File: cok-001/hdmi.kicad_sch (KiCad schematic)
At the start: 60 parts, among them J2501 HDMI_A, Q2502 DTA144E, Q2504 DTA144E, Q2507 DTC144E

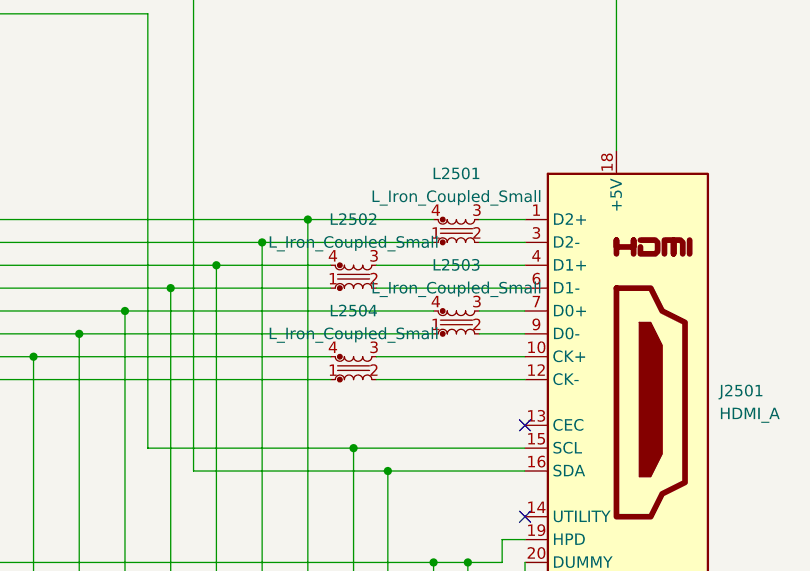
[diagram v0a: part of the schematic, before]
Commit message: ethernet
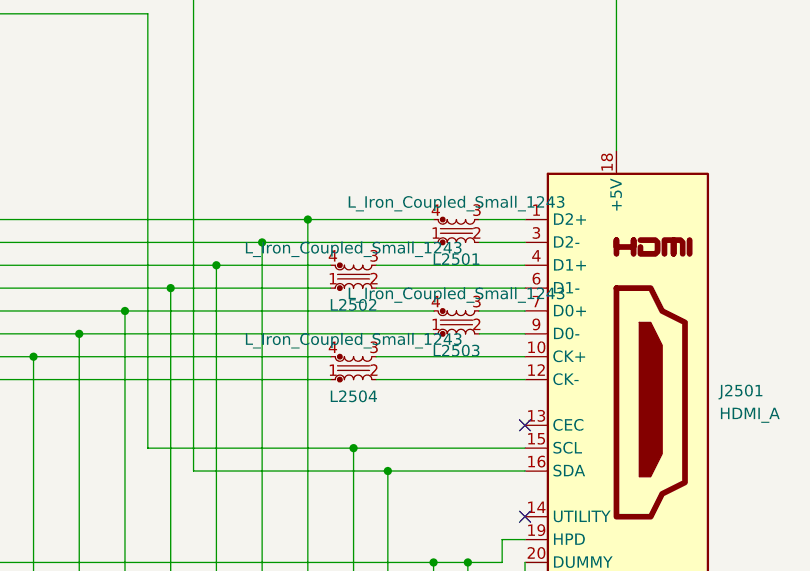
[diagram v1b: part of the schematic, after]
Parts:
- L2501, L2502, L2503, L2504: value L_Iron_Coupled_Small -> L_Iron_Coupled_Small_1243
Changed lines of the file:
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@@
 		(dnp no)
 		(property "Reference" "L2501"
-			(at 334.01 92.71 0)
+			(at 334.01 102.235 0)
 			(effects
 				(font
@@
 			)
 		)
-		(property "Value" "L_Iron_Coupled_Small"
-			(at 334.01 95.25 0)
+		(property "Value" "L_Iron_Coupled_Small_1243"
+			(at 334.01 95.885 0)
 			(effects
 				(font
@@
 		(dnp no)
 		(property "Reference" "L2502"
-			(at 322.58 97.79 0)
+			(at 322.58 107.315 0)
 			(effects
 				(font
@@
 			)
 		)
-		(property "Value" "L_Iron_Coupled_Small"
-			(at 322.58 100.33 0)
+		(property "Value" "L_Iron_Coupled_Small_1243"
+			(at 322.58 100.965 0)
 			(effects
 				(font
@@
 		(dnp no)
 		(property "Reference" "L2503"
-			(at 334.01 102.87 0)
+			(at 334.01 112.395 0)
 			(effects
 				(font
@@
 			)
 		)
-		(property "Value" "L_Iron_Coupled_Small"
-			(at 334.01 105.41 0)
+		(property "Value" "L_Iron_Coupled_Small_1243"
+			(at 334.01 106.045 0)
 			(effects
 				(font
@@
 		(dnp no)
 		(property "Reference" "L2504"
-			(at 322.58 107.95 0)
+			(at 322.58 117.475 0)
 			(effects
 				(font
@@
 			)
 		)
-		(property "Value" "L_Iron_Coupled_Small"
-			(at 322.58 110.49 0)
+		(property "Value" "L_Iron_Coupled_Small_1243"
+			(at 322.58 111.125 0)
 			(effects
 				(font

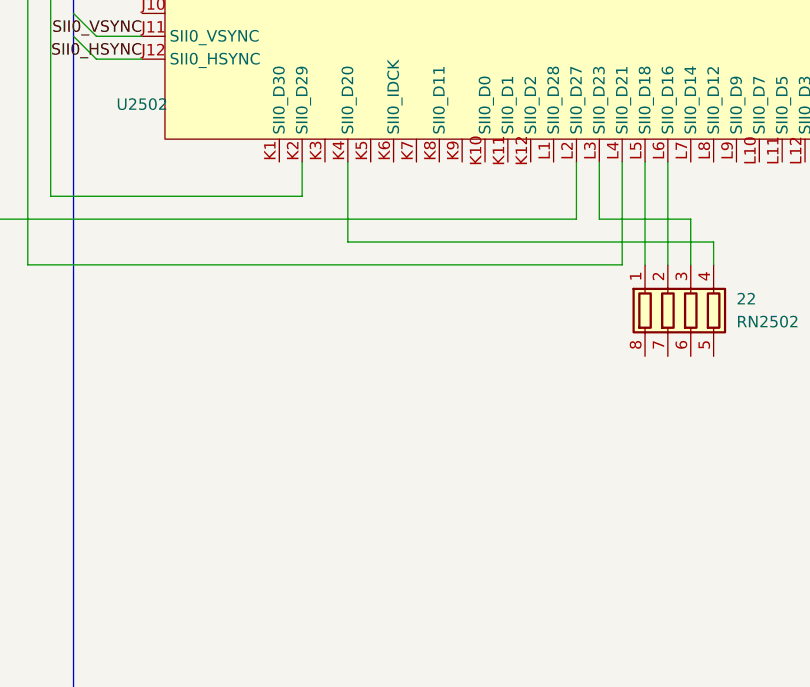
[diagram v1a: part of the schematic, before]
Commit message: sata
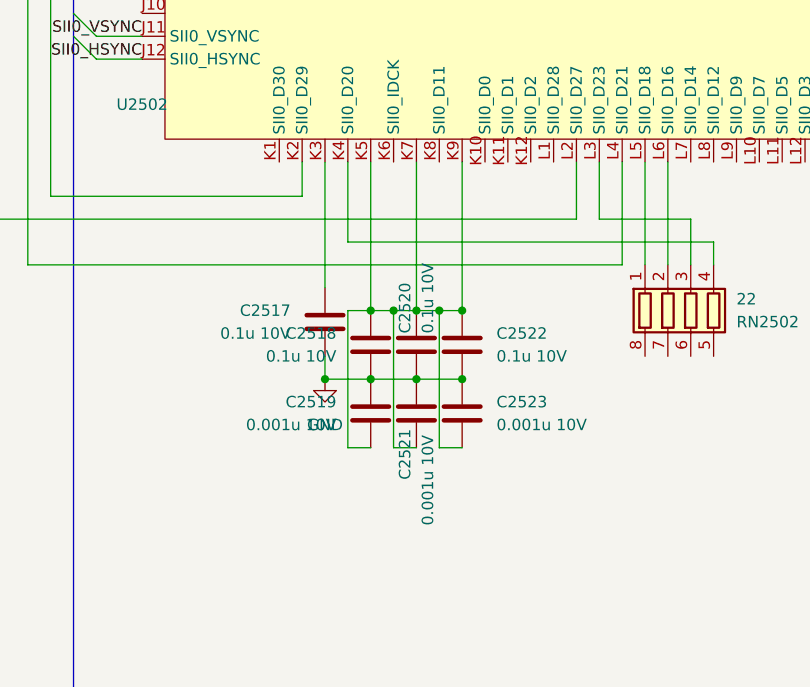
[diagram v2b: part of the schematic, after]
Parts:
- added C2517, C2518, C2520, C2522: 0.1u 10V, Capacitor_SMD:C_0402_1005Metric, symbol Device:C
- added C2519, C2521, C2523: 0.001u 10V, Capacitor_SMD:C_0402_1005Metric, symbol Device:C
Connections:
- net GND: now also C2517.2, C2518.2, C2519.1, C2520.2, C2521.1, C2522.2, C2523.1
- net at U2502.K3: now also C2517.1
- net at U2502.K5: now also U2502.K7, U2502.K9, C2518.1, C2519.2, C2520.1, C2521.2, C2522.1, C2523.2

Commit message: southbridge
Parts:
- D251, D252, D253, D254, D255, D256, D257, D258: footprint Diode_SMD:D_SOD-923 -> Diode_SMD:D_SOD-523
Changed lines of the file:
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@@
 			)
 		)
-		(property "Footprint" "Diode_SMD:D_SOD-923"
+		(property "Footprint" "Diode_SMD:D_SOD-523"
 			(at 282.575 147.32 0)
 			(effects
@@
 			)
 		)
-		(property "Footprint" "Diode_SMD:D_SOD-923"
+		(property "Footprint" "Diode_SMD:D_SOD-523"
 			(at 311.785 147.32 0)
 			(effects
@@
 			)
 		)
-		(property "Footprint" "Diode_SMD:D_SOD-923"
+		(property "Footprint" "Diode_SMD:D_SOD-523"
 			(at 287.655 147.32 0)
 			(effects
@@
 			)
 		)
-		(property "Footprint" "Diode_SMD:D_SOD-923"
+		(property "Footprint" "Diode_SMD:D_SOD-523"
 			(at 316.865 147.32 0)
 			(effects
@@
 			)
 		)
-		(property "Footprint" "Diode_SMD:D_SOD-923"
+		(property "Footprint" "Diode_SMD:D_SOD-523"
 			(at 292.735 147.32 0)
 			(effects
@@
 			)
 		)
-		(property "Footprint" "Diode_SMD:D_SOD-923"
+		(property "Footprint" "Diode_SMD:D_SOD-523"
 			(at 321.945 147.32 0)
 			(effects
@@
 			)
 		)
-		(property "Footprint" "Diode_SMD:D_SOD-923"
+		(property "Footprint" "Diode_SMD:D_SOD-523"
 			(at 306.705 147.32 0)
 			(effects
@@
 			)
 		)
-		(property "Footprint" "Diode_SMD:D_SOD-923"
+		(property "Footprint" "Diode_SMD:D_SOD-523"
 			(at 277.495 147.32 0)
 			(effects

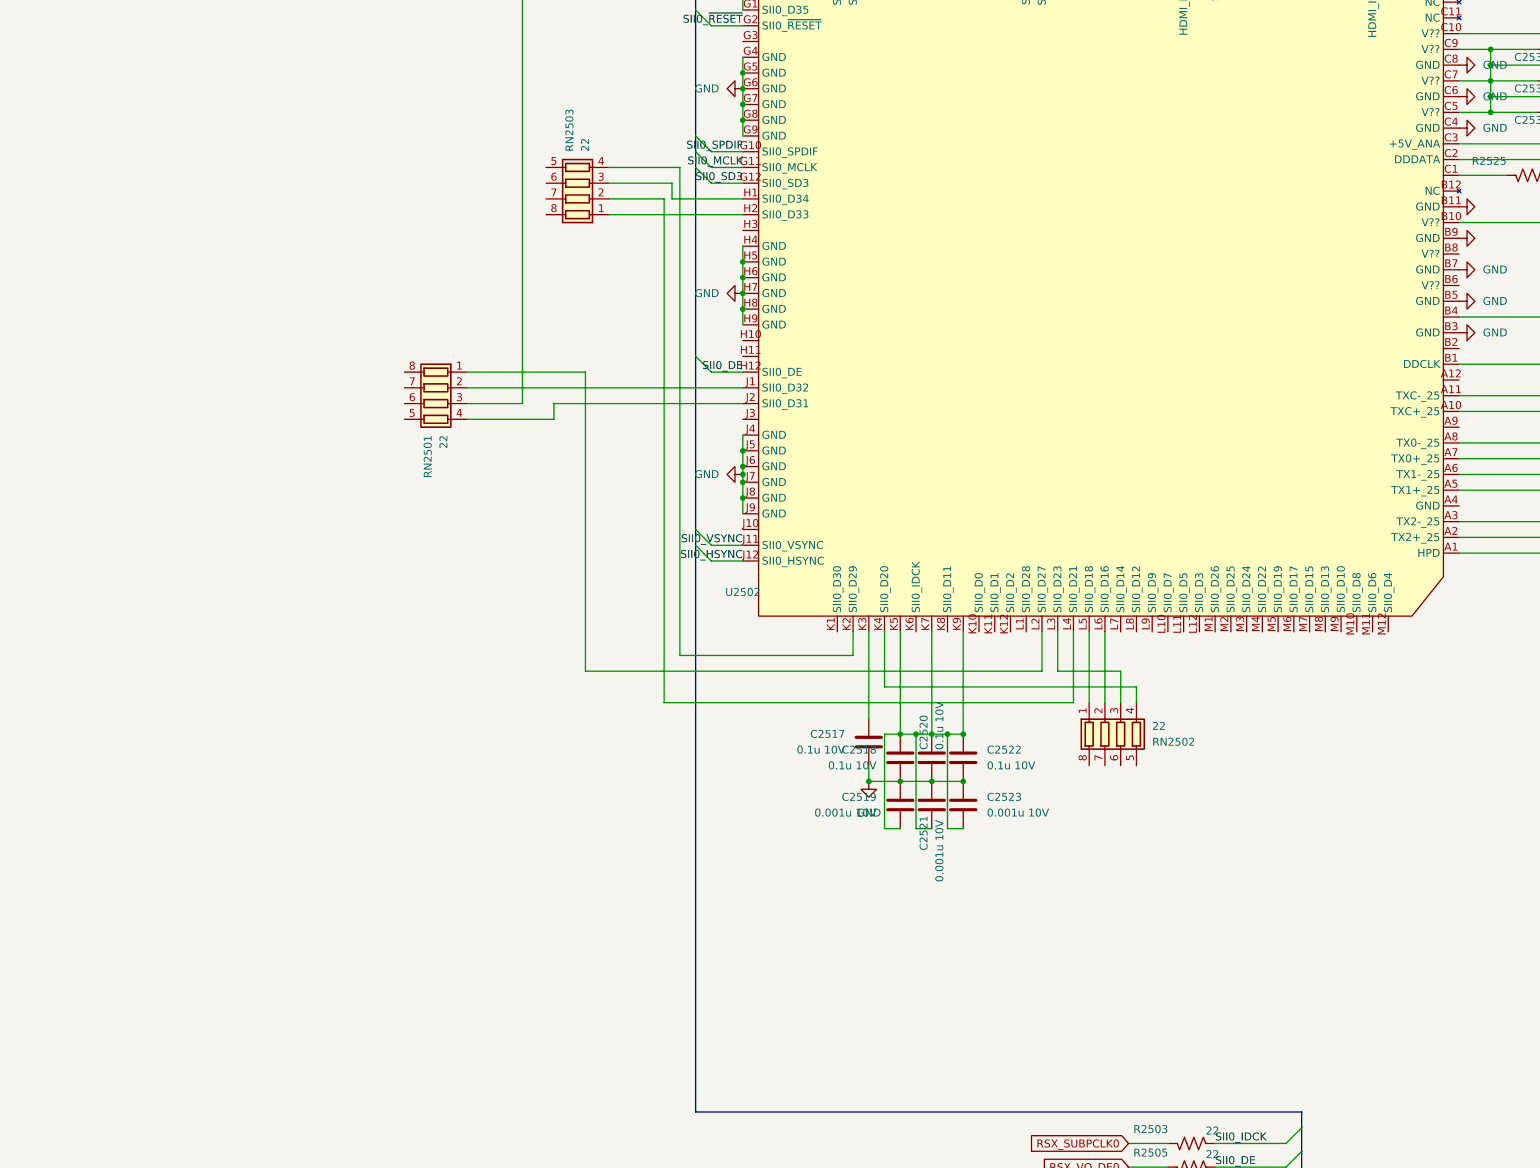
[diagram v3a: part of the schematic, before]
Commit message: aj
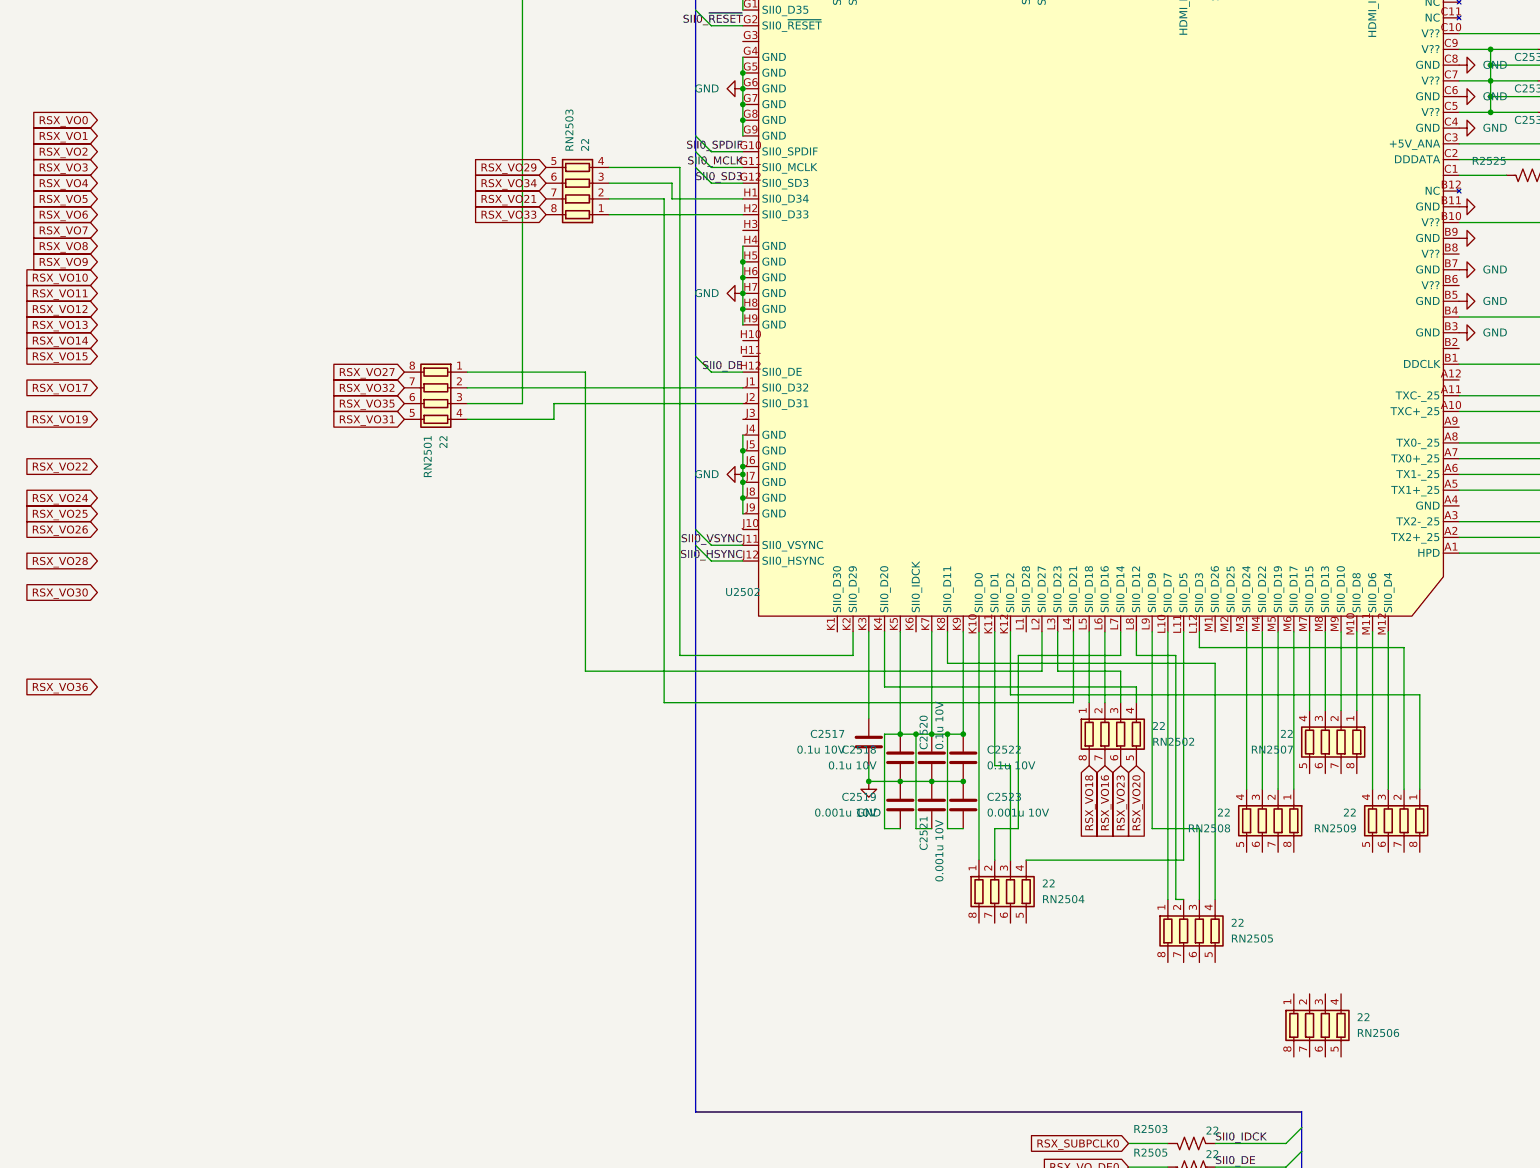
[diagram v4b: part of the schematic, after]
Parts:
- added RN2504, RN2505, RN2506, RN2507, RN2508, RN2509: 22, Resistor_SMD:R_Array_Convex_4x0402, symbol Device:R_Pack04
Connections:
- net RSX_VO29: now reaches RN2503.5 (R4.2)
- net RSX_VO34: now reaches RN2503.6 (R3.2)
- net RSX_VO21: now reaches RN2503.7 (R2.2)
- net RSX_VO33: now reaches RN2503.8 (R1.2)
- net RSX_VO20: now reaches RN2502.5 (R4.2)
- net RSX_VO23: now reaches RN2502.6 (R3.2)
- net RSX_VO16: now reaches RN2502.7 (R2.2)
- net RSX_VO18: now reaches RN2502.8 (R1.2)
- net at U2502.K10 (SII0_D0): now also RN2504.1 (R1.1)
- net at U2502.K11 (SII0_D1): now also RN2504.3 (R3.1)
- net at U2502.K12 (SII0_D2): now also RN2509.1 (R1.1)
- net at U2502.K8 (SII0_D11): now also RN2505.4 (R4.1)
- net at U2502.L10 (SII0_D7): now also RN2505.1 (R1.1)
- net at U2502.L11 (SII0_D5): now also RN2504.4 (R4.1)
- net at U2502.L12 (SII0_D3): now also RN2509.2 (R2.1)
- net at U2502.L7 (SII0_D14): now also RN2504.2 (R2.1)
- net at U2502.L8 (SII0_D12): now also RN2505.2 (R2.1)
- net at U2502.L9 (SII0_D9): now also RN2505.3 (R3.1)
- net at U2502.M10 (SII0_D8): now also RN2507.1 (R1.1)
- net at U2502.M11 (SII0_D6): now also RN2509.4 (R4.1)
- net at U2502.M12 (SII0_D4): now also RN2509.3 (R3.1)
- net at U2502.M3 (SII0_D24): now also RN2508.4 (R4.1)
- net at U2502.M4 (SII0_D22): now also RN2508.3 (R3.1)
- net at U2502.M5 (SII0_D19): now also RN2508.2 (R2.1)
- net at U2502.M6 (SII0_D17): now also RN2508.1 (R1.1)
- net at U2502.M7 (SII0_D15): now also RN2507.4 (R4.1)
- net at U2502.M8 (SII0_D13): now also RN2507.3 (R3.1)
- net at U2502.M9 (SII0_D10): now also RN2507.2 (R2.1)
- net RSX_VO31: now reaches RN2501.5 (R4.2)
- net RSX_VO35: now reaches RN2501.6 (R3.2)
- net RSX_VO32: now reaches RN2501.7 (R2.2)
- net RSX_VO27: now reaches RN2501.8 (R1.2)
